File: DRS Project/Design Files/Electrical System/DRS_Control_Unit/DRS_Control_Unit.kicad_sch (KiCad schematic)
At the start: 47 parts, among them IC1 AP63301QWU-7, J1 Screw, J2 Deutsch DT, J3 Servo, J4 DE9_Socket_MountingHoles, SW1 DSIC01THGET, U1 AMS1117, U2 Teensy4.0-NU-Teams, U3 TJA1051T-3, U4 LM2596S-ADJ

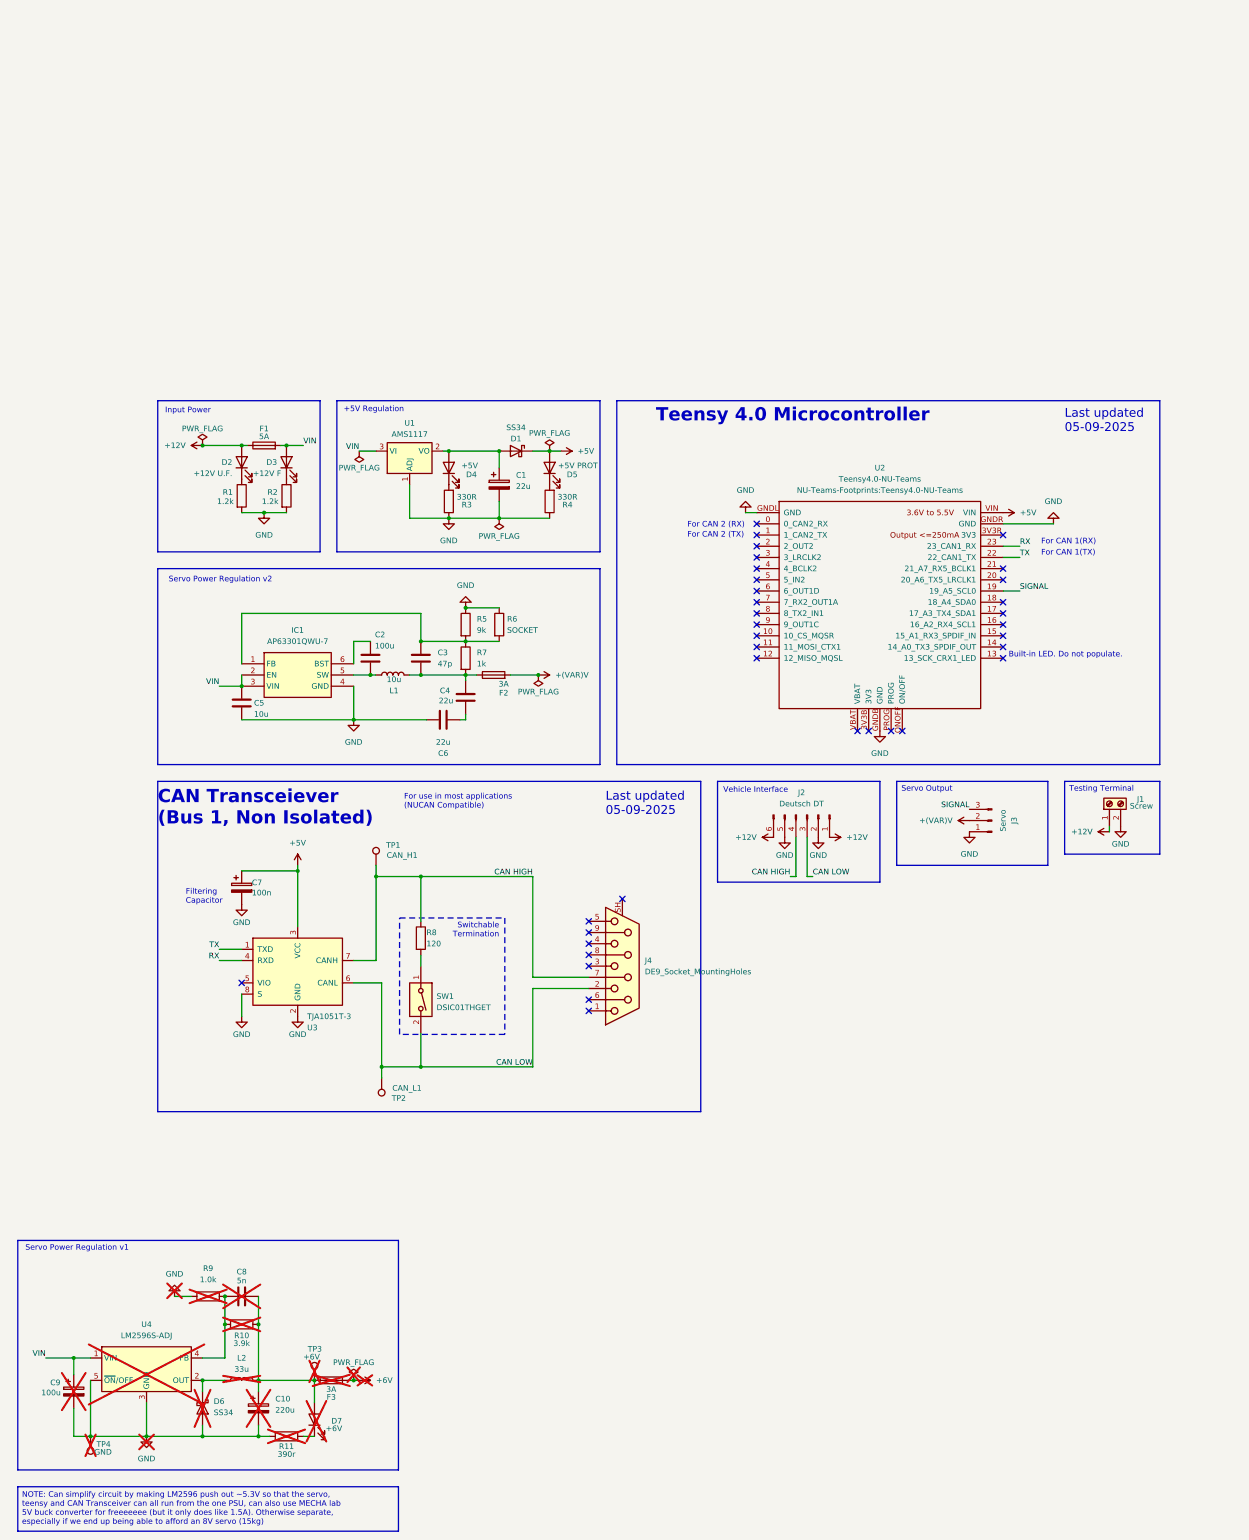
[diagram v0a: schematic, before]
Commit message: pcb rev 1 actually complete (fr this time)
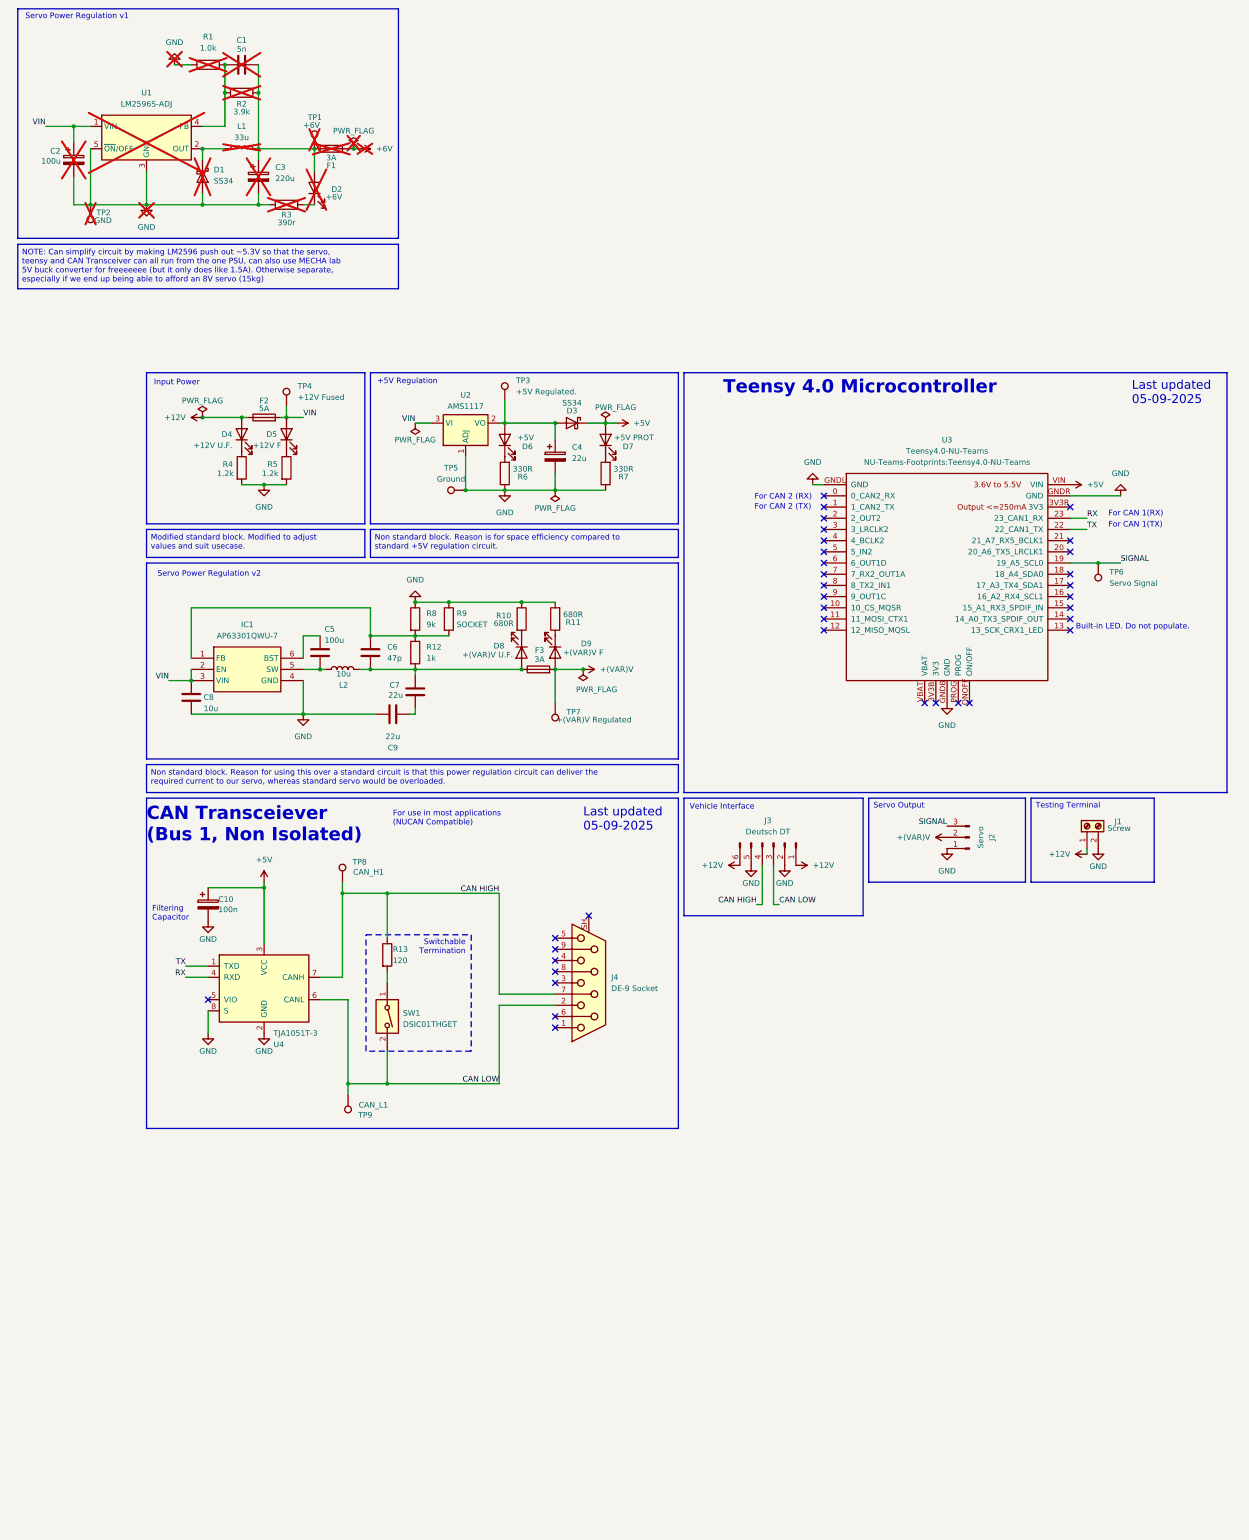
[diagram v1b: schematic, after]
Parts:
- added D8: +(VAR)V U.F., LED_SMD:LED_1206_3216Metric_Pad1.42x1.75mm_HandSolder, symbol Device:LED
- added D9: +(VAR)V F, LED_SMD:LED_1206_3216Metric_Pad1.42x1.75mm_HandSolder, symbol Device:LED
- added R10, R11: 680R, Resistor_SMD:R_1206_3216Metric_Pad1.30x1.75mm_HandSolder, symbol Device:R
- added TP3: +5V Regulated., TestPoint:TestPoint_Loop_D1.80mm_Drill1.0mm_Beaded, symbol Connector:TestPoint
- added TP4: +12V Fused, TestPoint:TestPoint_Loop_D1.80mm_Drill1.0mm_Beaded, symbol Connector:TestPoint
- added TP5: Ground, TestPoint:TestPoint_Loop_D1.80mm_Drill1.0mm_Beaded, symbol Connector:TestPoint
- added TP6: Servo Signal, TestPoint:TestPoint_Loop_D1.80mm_Drill1.0mm_Beaded, symbol Connector:TestPoint
- added TP7: +(VAR)V Regulated, TestPoint:TestPoint_Loop_D1.80mm_Drill1.0mm_Beaded, symbol Connector:TestPoint
- J4: value DE9_Socket_MountingHoles -> DE-9 Socket
- renumbered C8 to C1, C7 to C10, C9 to C2, C10 to C3, C1 to C4, C2 to C5, C3 to C6, C4 to C7, C5 to C8, C6 to C9, D6 to D1, D7 to D2, D1 to D3, D2 to D4, D3 to D5, D4 to D6, D5 to D7, F3 to F1, F1 to F2, F2 to F3, J3 to J2, J2 to J3, L2 to L1, L1 to L2, R9 to R1, R7 to R12, R8 to R13, R10 to R2, R11 to R3, R1 to R4, R2 to R5, R3 to R6, R4 to R7, R5 to R8, R6 to R9, TP3 to TP1, TP4 to TP2, TP1 to TP8, TP2 to TP9, U4 to U1, U1 to U2, U2 to U3, U3 to U4
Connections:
- net +(VAR)V: now also D9.2 (A), TP7.1
- net GND: now also R10.1, R11.2, TP5.1
- net SIGNAL: now also TP6.1
- net VIN: now also TP4.1
- net at C4.1, D3.2 (A), D6.2 (A)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: now also TP3.1
- net at C6.2, C7.1, F3.1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: now also D8.2 (A)
- new net: D9.1 (K), R11.1
- new net: D8.1 (K), R10.2
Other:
- moved on the sheet: C1, C10, C2, C3, C4, C5, C6, C7, C8, C9, D1, D2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
